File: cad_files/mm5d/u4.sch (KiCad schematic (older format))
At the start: 30 parts, among them SW401 SWITCH_1P

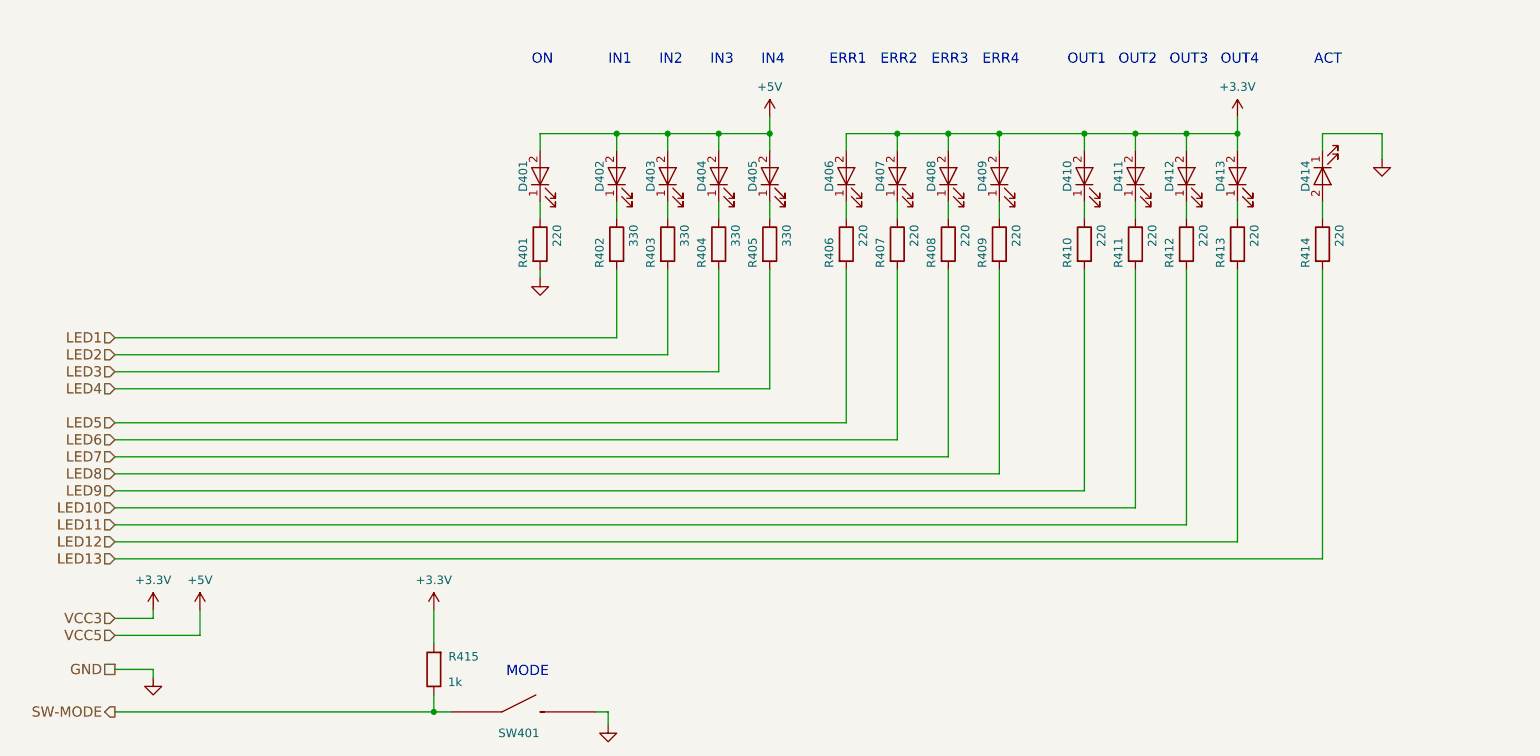
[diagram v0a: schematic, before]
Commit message: 200129
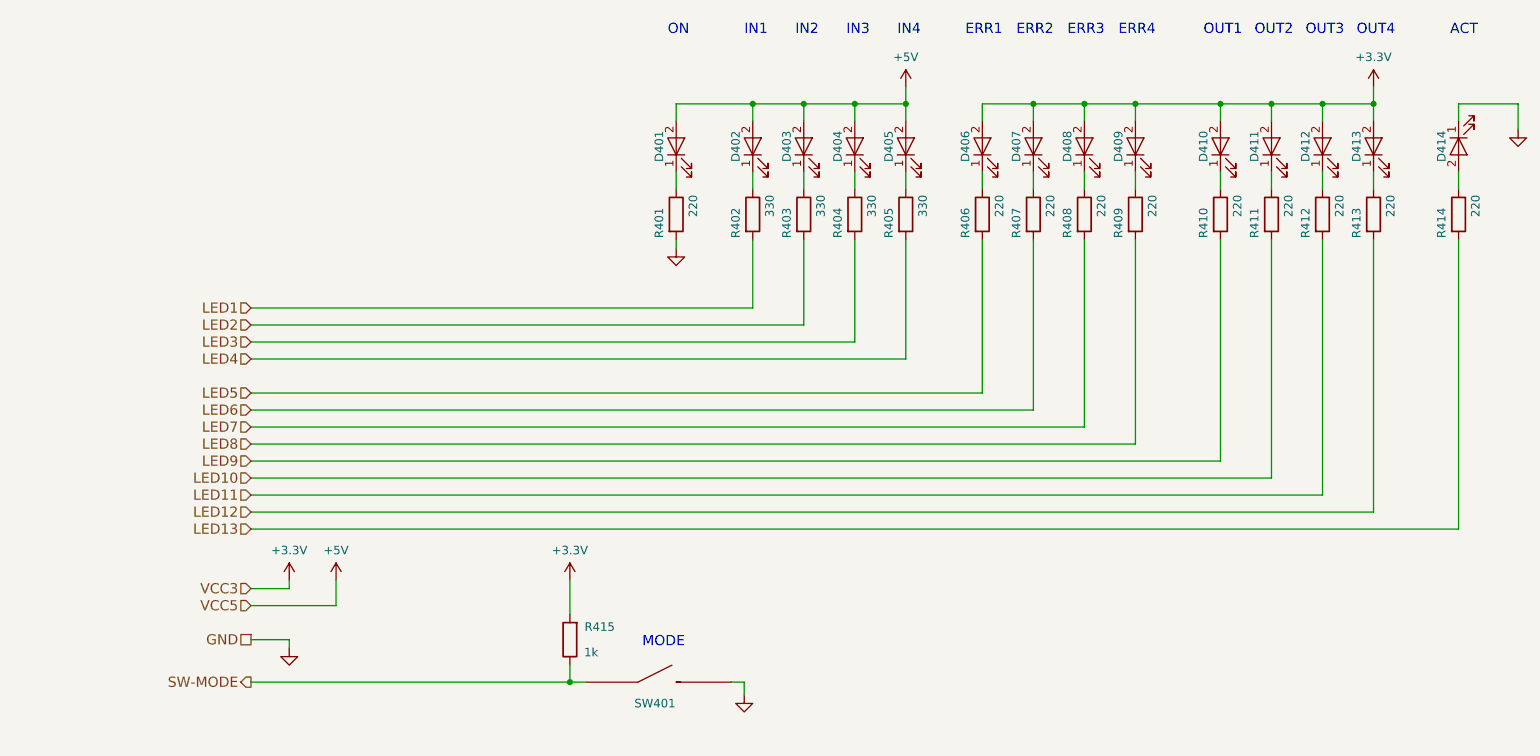
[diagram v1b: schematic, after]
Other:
- moved on the sheet: D401, D402, D403, D404, D405, D406, D407, D408, D409, D410, D411, D412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

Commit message: 200130
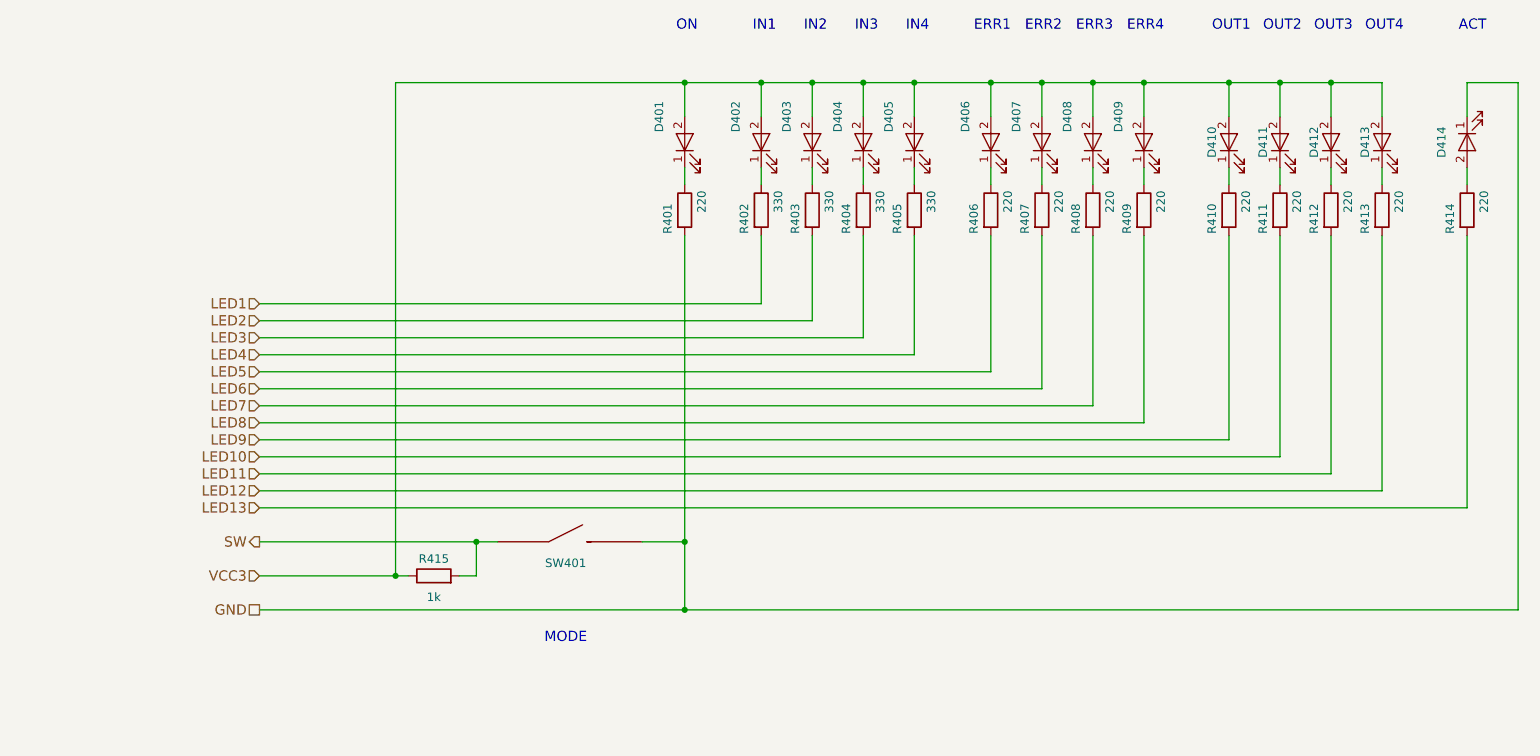
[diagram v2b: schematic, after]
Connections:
- net +5V is gone; now on net VCC3: D401.2 (A), D402.2 (A), D403.2 (A), D404.2 (A), D405.2 (A)
- net +3V3 renamed VCC3
- net VCC3: now also R415.1; no longer R415.2
- net SW-MODE renamed SW
- net SW: now also R415.2; no longer R415.1
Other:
- moved on the sheet: D401, D402, D403, D404, D405, D406, D407, D408, D409, D410, D411, D412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
